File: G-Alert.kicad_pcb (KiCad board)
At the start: 2 copper layers, 39.1 x 91.4 mm, 19 parts, among them SW1 SW_Push, U1 MQ-4b, U2 LM393

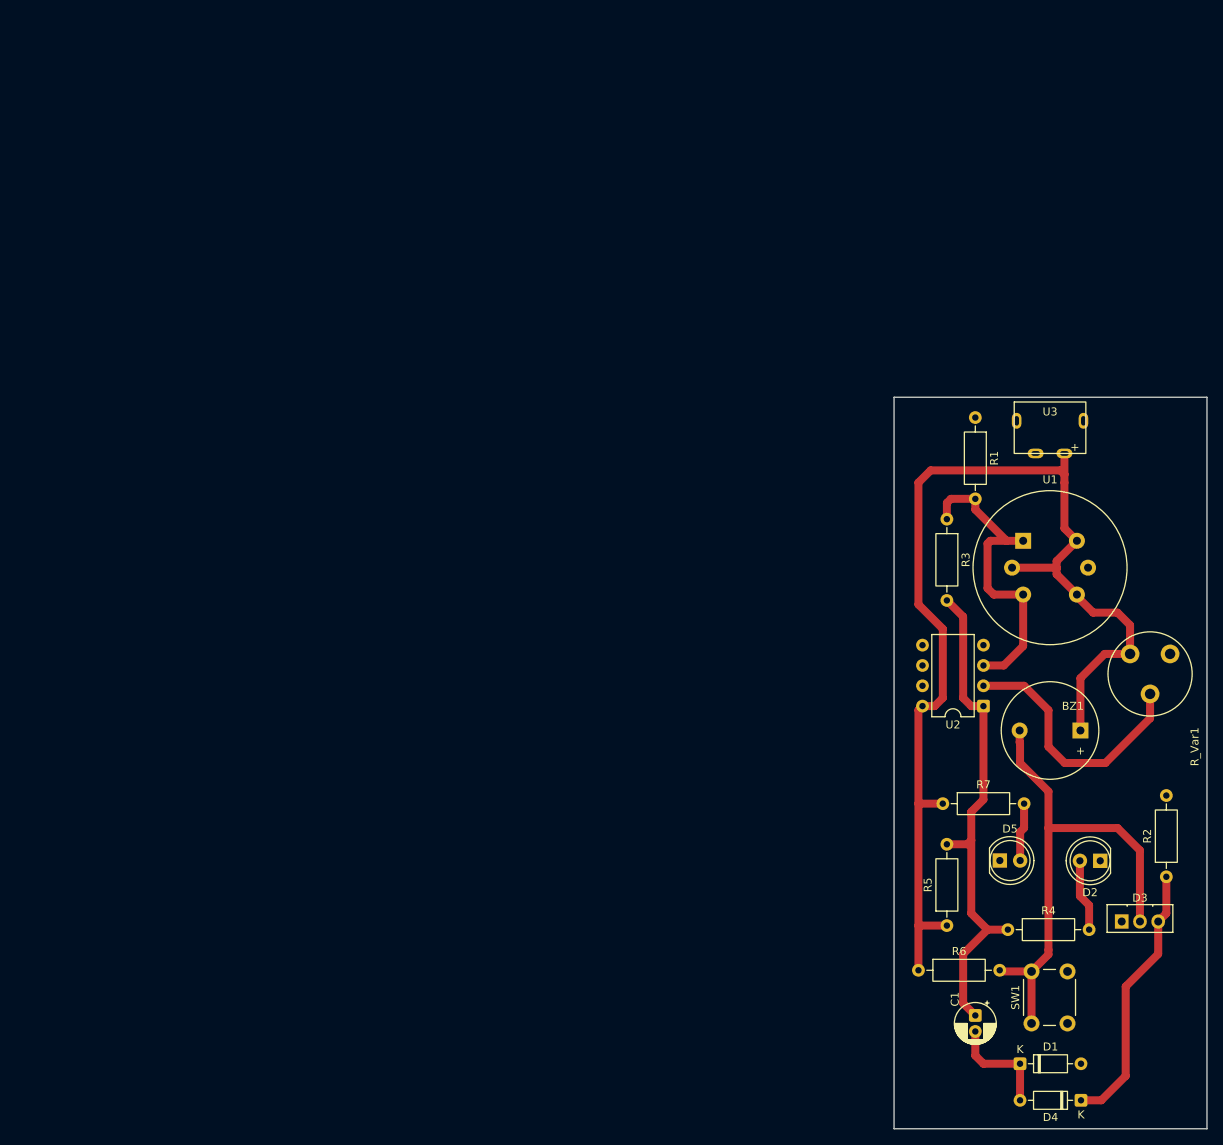
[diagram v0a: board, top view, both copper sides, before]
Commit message: pcb-semifinal
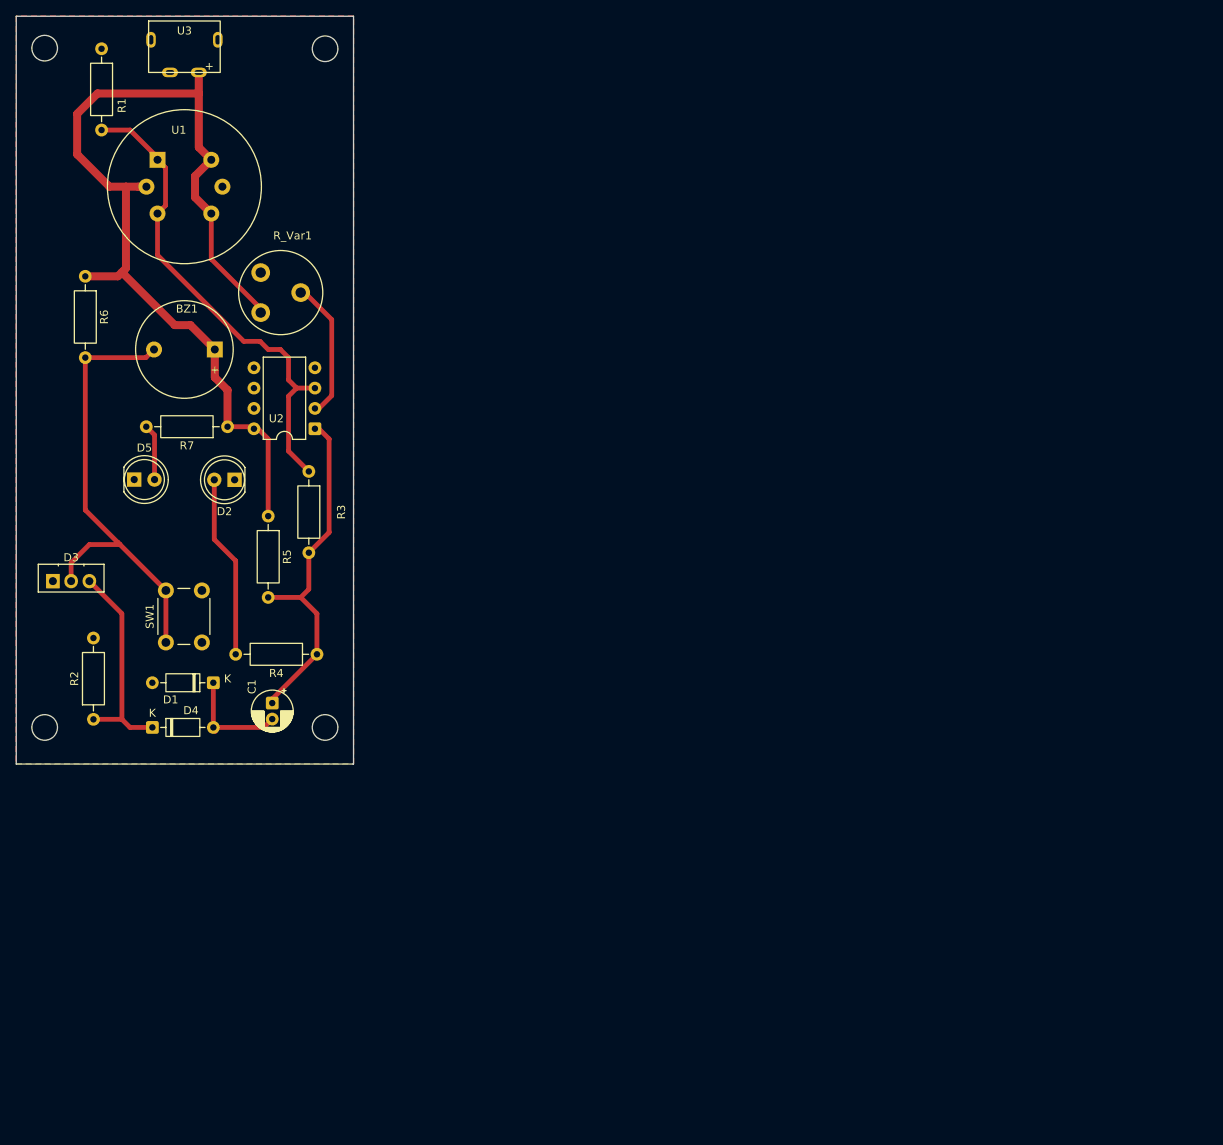
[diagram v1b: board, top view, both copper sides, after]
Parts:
- moved D3 140.2 mm to (25.4, 90.0)
- moved R2 135.5 mm to (30.5, 107.3)
- moved R6 135.5 mm to (29.5, 51.9), turned to -90 degrees
- moved D4 125.1 mm to (37.8, 108.3), turned to 0 degrees
- moved R1 118.6 mm to (31.5, 23.5)
- moved D2 118.2 mm to (48.1, 77.4)
- moved D5 118.2 mm to (35.6, 77.3)
- moved SW1 118.2 mm to (39.5, 97.7)
- moved U3 118.2 mm to (41.9, 22.4)
- moved U1 118.2 mm to (38.5, 37.4)
- moved BZ1 118.2 mm to (45.7, 61.1)
- moved R_Var1 116.7 mm to (51.4, 56.5), turned to 0 degrees
- moved D1 111.5 mm to (45.5, 102.7), turned to 180 degrees
- moved R7 101.1 mm to (47.2, 70.7), turned to 180 degrees
- moved R5 99.1 mm to (52.3, 81.9), turned to -90 degrees
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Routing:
- net Net-(U1-B1): track 40.0 -> 61.5 mm
- net Net-(C1-Pad1): track 63.8 -> 43.5 mm
- net +5V: track 142.3 -> 123.8 mm
- net Net-(U2A--): track 32.9 -> 17.0 mm
- net Net-(D2-A): track 9.08 -> 22.9 mm
- net Net-(D3-G): track 33.8 -> 26.7 mm
- net Net-(BZ1--): track 64.5 -> 58.5 mm
- net Net-(D1-K): track 13.6 -> 14.3 mm
- added copper zone on F.Cu, net GND
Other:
- board size 39.1 x 91.4 mm -> 42.2 x 93.5 mm
